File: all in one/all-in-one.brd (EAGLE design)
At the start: 100 x 80 mm, 89 parts, among them J1 K1, J10 DIN, J11 START, J12 SELECT, J13 HOME, J14 BALLTOP, J15 PLATE, J2 P1, J20 DOUT, J21 led, J3 K2, J4 P2, J5 K3, J6 P3, J7 K4, J8 P4, J9 led

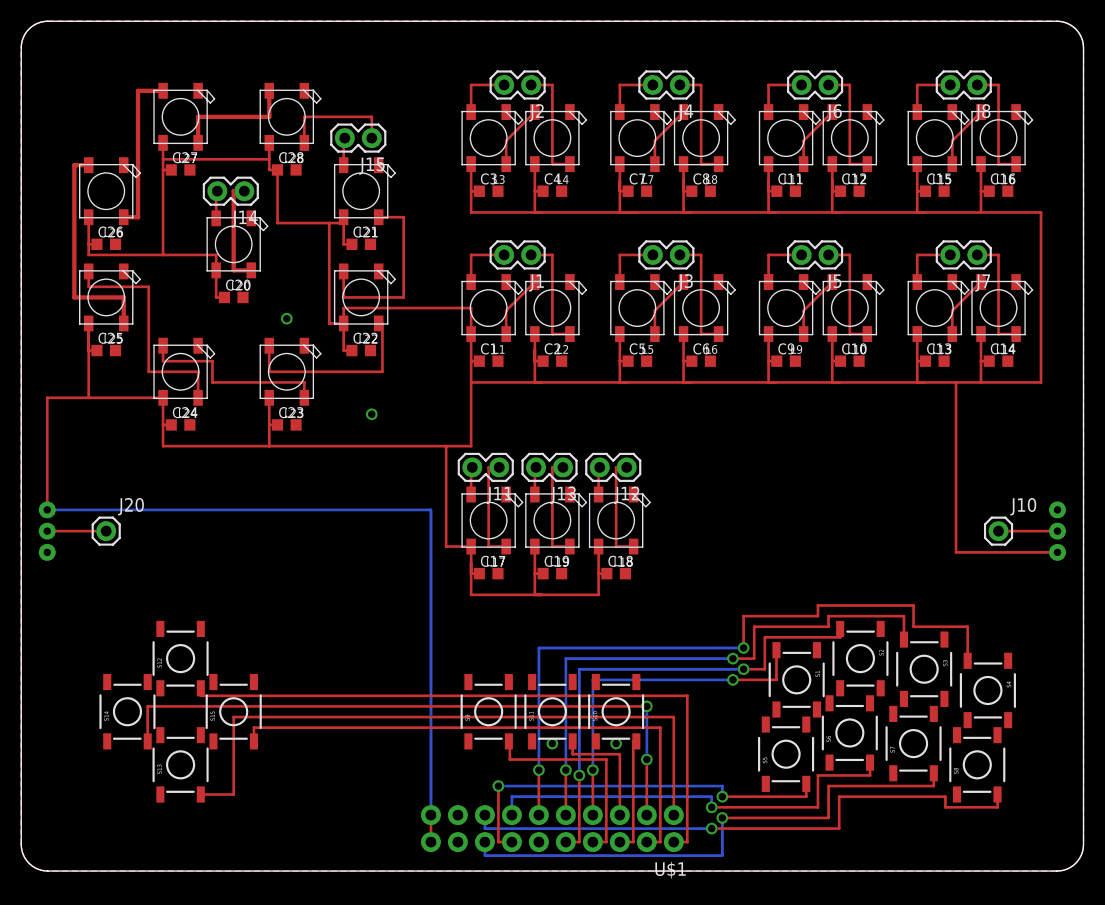
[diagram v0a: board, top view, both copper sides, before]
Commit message: rooby dooby dooby
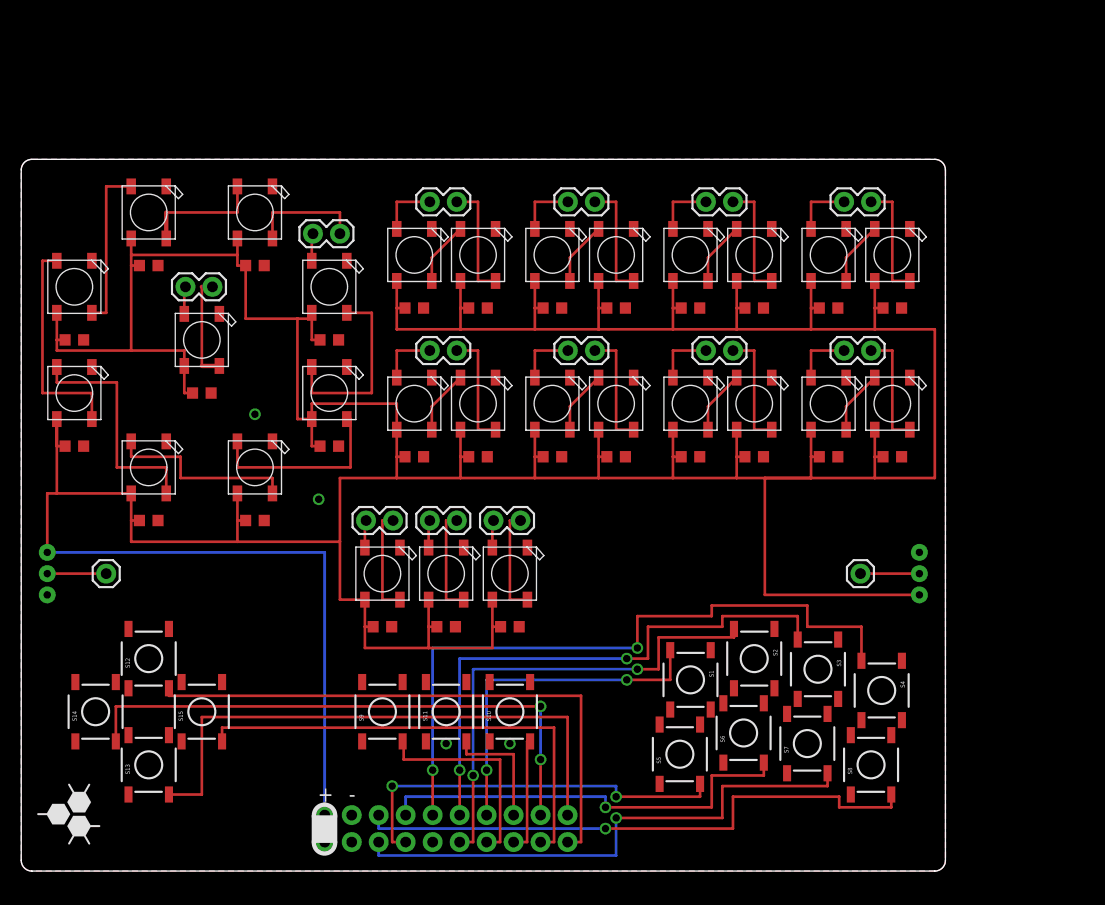
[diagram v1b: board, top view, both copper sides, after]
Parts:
- moved C15 14.9 mm to (76.0, 53.0)
- moved C16 14.9 mm to (82.0, 53.0)
- moved J8 14.9 mm to (80.0, 63.0)
- moved L15 14.9 mm to (76.0, 58.0)
- moved L16 14.9 mm to (82.0, 58.0)
- moved C11 14.2 mm to (63.0, 53.0)
- moved C12 14.2 mm to (69.0, 53.0)
- moved J6 14.2 mm to (67.0, 63.0)
- moved L11 14.2 mm to (63.0, 58.0)
- moved L12 14.2 mm to (69.0, 58.0)
- moved C7 13.6 mm to (50.0, 53.0)
- moved C8 13.6 mm to (56.0, 53.0)
- moved J10 13.6 mm to (79.0, 28.0)
- moved J4 13.6 mm to (54.0, 63.0)
- moved J9 13.6 mm to (84.0, 28.0)
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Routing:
- net VCC: track 524.4 -> 471.3 mm
- net UP: track 61.5 -> 54.5 mm
- net RIGHT: track 51.6 -> 44.6 mm
- net LEFT: track 60.5 -> 53.5 mm
- net DOWN: track 61.0 -> 54.0 mm
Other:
- board size 100 x 80 mm -> 87 x 67 mm
- board text added: "+"
- board text added: "-"
- board text added: "1P ST"
- board text added: "2K 1K"
- board text added: "3P 2P"
- board text added: "4K 3K"
- board text added: "4P -"
- board text added: "BALL"
- board text added: "DN UP"
- board text added: "HO SE"
- board text added: "HOME"
- board text added: "K1"
- board text added: "K2"
- board text added: "K3"
- board text added: "K4"
- board text added: "LT RT"
- board text added: "P1"
- board text added: "P2"
- board text added: "P3"
- board text added: "P4"
- board text added: "PLATE"
- board text added: "SEL"
- board text added: "STA"
